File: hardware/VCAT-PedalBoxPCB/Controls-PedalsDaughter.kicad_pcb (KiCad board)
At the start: 2 copper layers, 53 x 66.2 mm, 105 parts, among them IC1 AP2205-W5-7, IC2 AP2205-W5-7, J3 Conn_02x03_Top_Bottom, J4 Conn_02x06_Top_Bottom, J5 Conn_02x04_Top_Bottom, U1 TLV9002QDRQ1, U2 INA241A5xD, U3 TLV9002QDRQ1, U4 INA241A5xD, U5 TLV9002QDRQ1

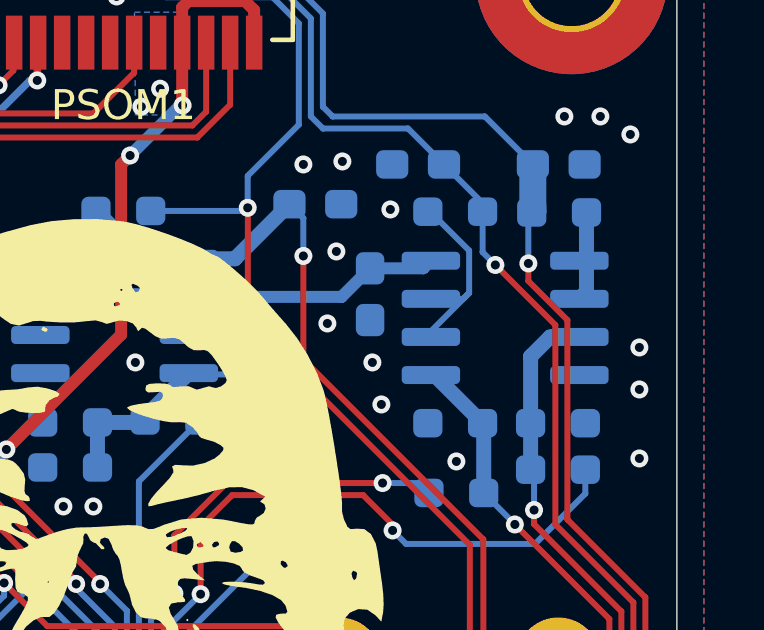
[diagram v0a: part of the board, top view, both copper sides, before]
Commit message: lcsc + prod files
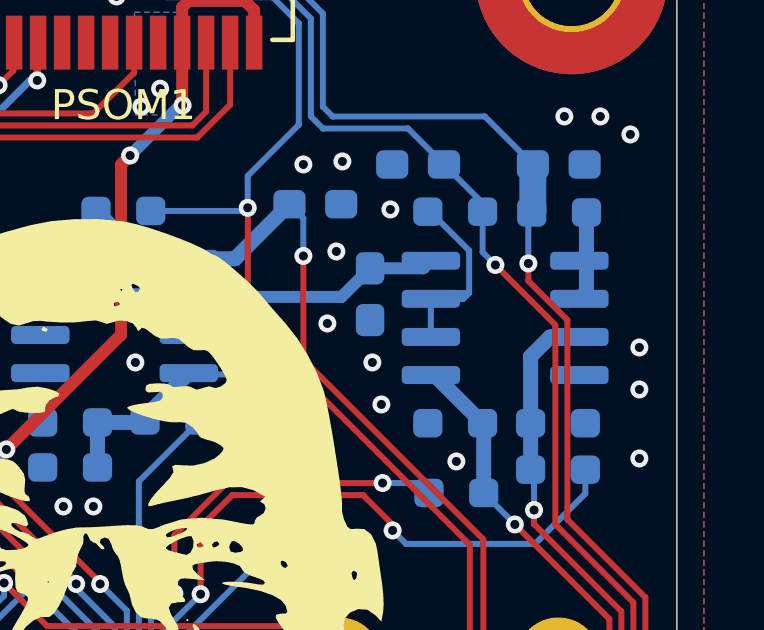
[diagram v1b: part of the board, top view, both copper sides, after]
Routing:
- net /Pedals/Dual Op Amp Buffer Pots (main)/In2-: track 6.68 -> 7.31 mm
